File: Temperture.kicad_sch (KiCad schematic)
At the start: 6 parts

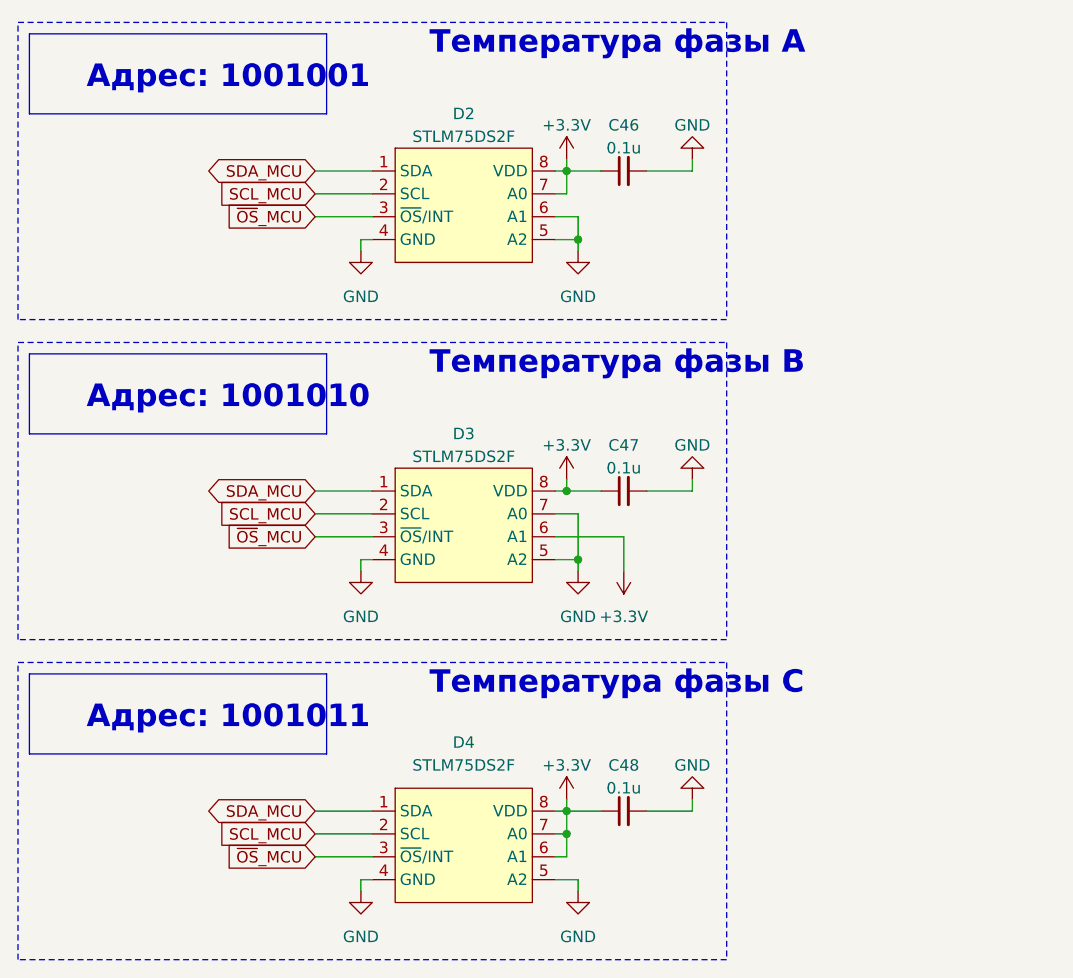
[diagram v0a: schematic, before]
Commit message: Первый вариант
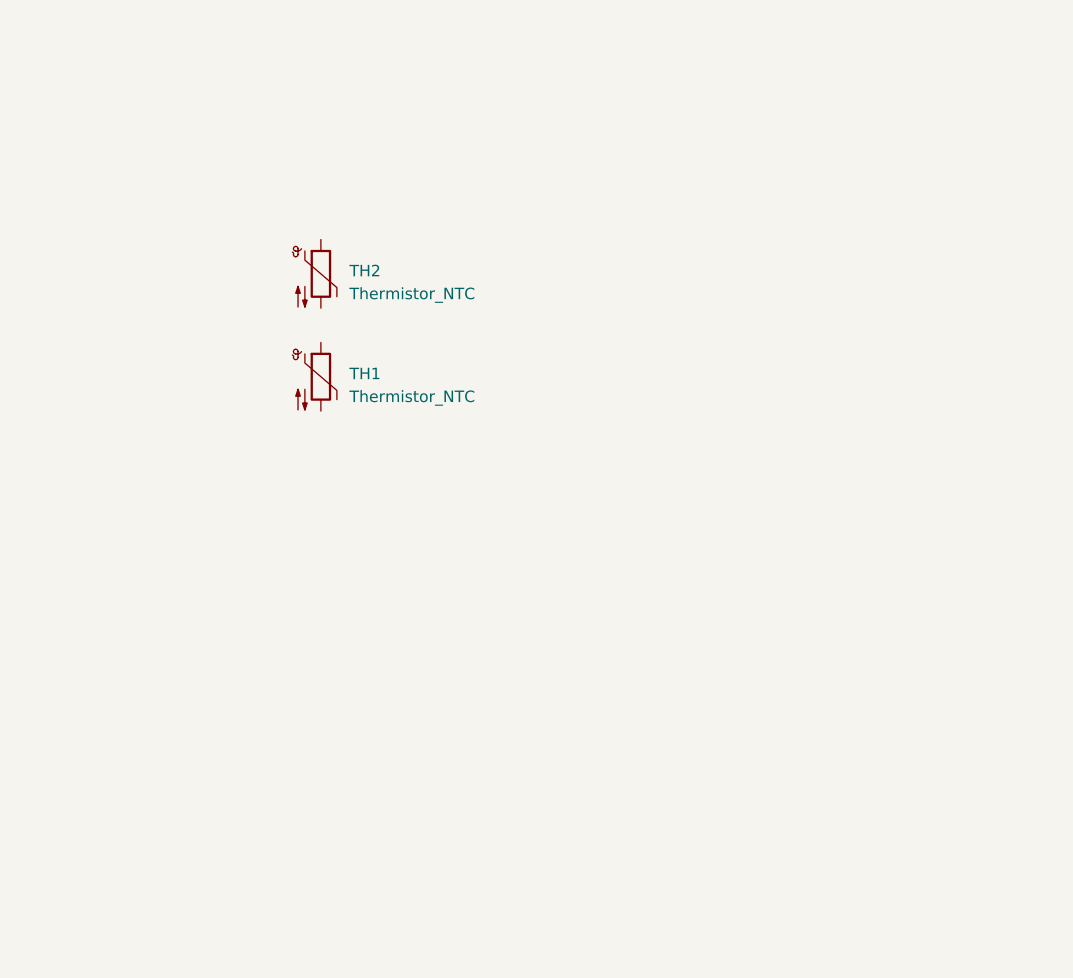
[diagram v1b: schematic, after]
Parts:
- removed C46, C47, C48: 0.1u, Capacitor_SMD:C_0603_1608Metric_Pad1.08x0.95mm_HandSolder, symbol Device:C_Small
- removed D2, D3, D4: STLM75DS2F, Package_SO:MSOP-8_3x3mm_P0.65mm, symbol Temperature_My:STLM75DS2F
- added TH1, TH2: Thermistor_NTC, symbol Device:Thermistor_NTC
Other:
- note removed: "Адрес: 1001001"
- note removed: "Адрес: 1001010"
- note removed: "Адрес: 1001011"
- note removed: "Температура фазы А"
- note removed: "Температура фазы В"
- note removed: "Температура фазы С"

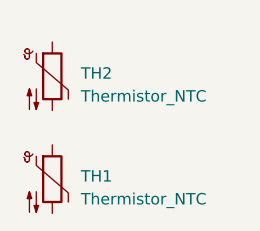
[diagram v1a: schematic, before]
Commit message: Сохранил схему
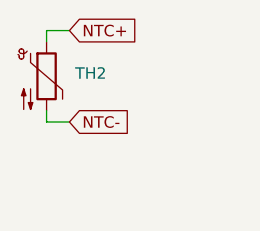
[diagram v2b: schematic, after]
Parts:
- removed TH1: Thermistor_NTC, symbol Device:Thermistor_NTC
- TH2: footprint (none) -> Resistor_SMD:R_0603_1608Metric_Pad0.98x0.95mm_HandSolder
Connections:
- net NTC+: now reaches TH2.1
- net NTC-: now reaches TH2.2
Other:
- moved on the sheet: TH2
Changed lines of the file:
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@@
-(kicad_sch (version 20230121) (generator eeschema)
-  (paper "A4")
-  (title_block
-    (company "Московский Политех")
-    (comment 1 "МПСТ.76721.758764.01.М Э3")
-  )
-  (symbol (lib_id "Device:Thermistor_NTC") (at 145.415 87.63 0) (unit 1)
-    (in_bom yes) (on_board yes) (dnp no) (fields_autoplaced)
-    (property "Reference" "TH1" (at 148.59 87.3124 0)
-      (effects (font (size 1.27 1.27)) (justify left))
-    )
-    (property "Value" "Thermistor_NTC" (at 148.59 89.8524 0)
-      (effects (font (size 1.27 1.27)) (justify left))
-    )
-    (property "Footprint" "" (at 145.415 86.36 0)
-      (effects (font (size 1.27 1.27)) hide)
-    )
-    (property "Datasheet" "~" (at 145.415 86.36 0)
-      (effects (font (size 1.27 1.27)) hide)
-    )
-    (pin "1")
-    (pin "2")
-    (instances
-      (project "Силовая плата"
-        (path "/96c6fc92-8ec6-44f7-b0dc-9ad8f1acea09/005a885b-ef5f-4b8c-934f-72ceac7d73e5"
-          (reference "TH1") (unit 1)
-        )
-      )
-    )
-  )
-  (symbol (lib_id "Device:Thermistor_NTC") (at 145.415 76.2 0) (unit 1)
-    (in_bom yes) (on_board yes) (dnp no) (fields_autoplaced)
-    (property "Reference" "TH2" (at 148.59 75.8824 0)
-      (effects (font (size 1.27 1.27)) (justify left))
-    )
-    (property "Value" "Thermistor_NTC" (at 148.59 78.4224 0)
-      (effects (font (size 1.27 1.27)) (justify left))
-    )
-    (property "Footprint" "" (at 145.415 74.93 0)
-      (effects (font (size 1.27 1.27)) hide)
-    )
-    (property "Datasheet" "~" (at 145.415 74.93 0)
-      (effects (font (size 1.27 1.27)) hide)
-    )
-    (pin "1")
-    (pin "2")
-    (instances
-      (project "Силовая плата"
-        (path "/96c6fc92-8ec6-44f7-b0dc-9ad8f1acea09/005a885b-ef5f-4b8c-934f-72ceac7d73e5"
-          (reference "TH2") (unit 1)
-        )
-      )
-    )
-  )
+(kicad_sch
+	(version 20231120)
+	(generator "eeschema")
+	(generator_version "8.0")
+	(paper "A4")
+	(title_block
+		(company "Московский Политех")
+		(comment 1 "МПСТ.76721.758764.01.М Э3")
+	)
+	(wire
+		(pts
+			(xy 144.78 80.01) (xy 144.78 81.28)
+		)
+		(stroke
+			(width 0)
+			(type default)
+		)
+	)
+	(wire
+		(pts
+			(xy 144.78 71.12) (xy 147.32 71.12)
+		)
+		(stroke
+			(width 0)
+			(type default)
+		)
+	)
+	(wire
+		(pts
+			(xy 144.78 71.12) (xy 144.78 72.39)
+		)
+		(stroke
+			(width 0)
+			(type default)
+		)
+	)
+	(wire
+		(pts
+			(xy 144.78 81.28) (xy 147.32 81.28)
+		)
+		(stroke
+			(width 0)
+			(type default)
+		)
+	)
+	(global_label "NTC-"
+		(shape input)
+		(at 147.32 81.28 0)
+		(fields_autoplaced yes)
+		(effects
+			(font
+				(size 1.27 1.27)
+			)
+			(justify left)
+		)
+		(property "Intersheetrefs" "${INTERSHEET_REFS}"
+			(at 153.8968 81.28 0)
+			(effects
+				(font
+					(size 1.27 1.27)
+				)
+				(justify left)
+				(hide yes)
+			)
+		)
+	)
+	(global_label "NTC+"
+		(shape input)
+		(at 147.32 71.12 0)
+		(fields_autoplaced yes)
+		(effects
+			(font
+				(size 1.27 1.27)
+			)
+			(justify left)
+		)
+		(property "Intersheetrefs" "${INTERSHEET_REFS}"
+			(at 153.8968 71.12 0)
+			(effects
+				(font
+					(size 1.27 1.27)
+				)
+				(justify left)
+				(hide yes)
+			)
+		)
+	)
+	(symbol
+		(lib_id "Device:Thermistor_NTC")
+		(at 144.78 76.2 0)
+		(unit 1)
+		(exclude_from_sim no)
+		(in_bom yes)
+		(on_board yes)
+		(dnp no)
+		(fields_autoplaced yes)
+		(property "Reference" "TH2"
+			(at 147.955 75.8824 0)
+			(effects
+				(font
+					(size 1.27 1.27)
+				)
+				(justify left)
+			)
+		)
+		(property "Value" "Thermistor_NTC"
+			(at 147.955 78.4224 0)
+			(effects
+				(font
+					(size 1.27 1.27)
+				)
+				(justify left)
+				(hide yes)
+			)
+		)
+		(property "Footprint" "Resistor_SMD:R_0603_1608Metric_Pad0.98x0.95mm_HandSolder"
+			(at 144.78 74.93 0)
+			(effects
+				(font
+					(size 1.27 1.27)
+				)
+				(hide yes)
+			)
+		)
+		(property "Datasheet" "~"
+			(at 144.78 74.93 0)
+			(effects
+				(font
+					(size 1.27 1.27)
+				)
+				(hide yes)
+			)
+		)
+		(property "Description" ""
+			(at 144.78 76.2 0)
+			(effects
+				(font
+					(size 1.27 1.27)
+				)
+				(hide yes)
+			)
+		)
+		(pin "1"
+		)
+		(pin "2"
+		)
+		(instances
+			(project "Силовая плата"
+				(path "/96c6fc92-8ec6-44f7-b0dc-9ad8f1acea09/005a885b-ef5f-4b8c-934f-72ceac7d73e5"
+					(reference "TH2")
+					(unit 1)
+				)
+			)
+		)
+	)
 )
